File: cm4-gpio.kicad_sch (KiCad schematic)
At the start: 28 parts, among them J1 B2B-PH-SM4-TB_LF__SN_, J5 Conn_02x05_Odd_Even, J6 USB4105-GF-A, U1 MP2624GL-P, U2 MP3423GG-P

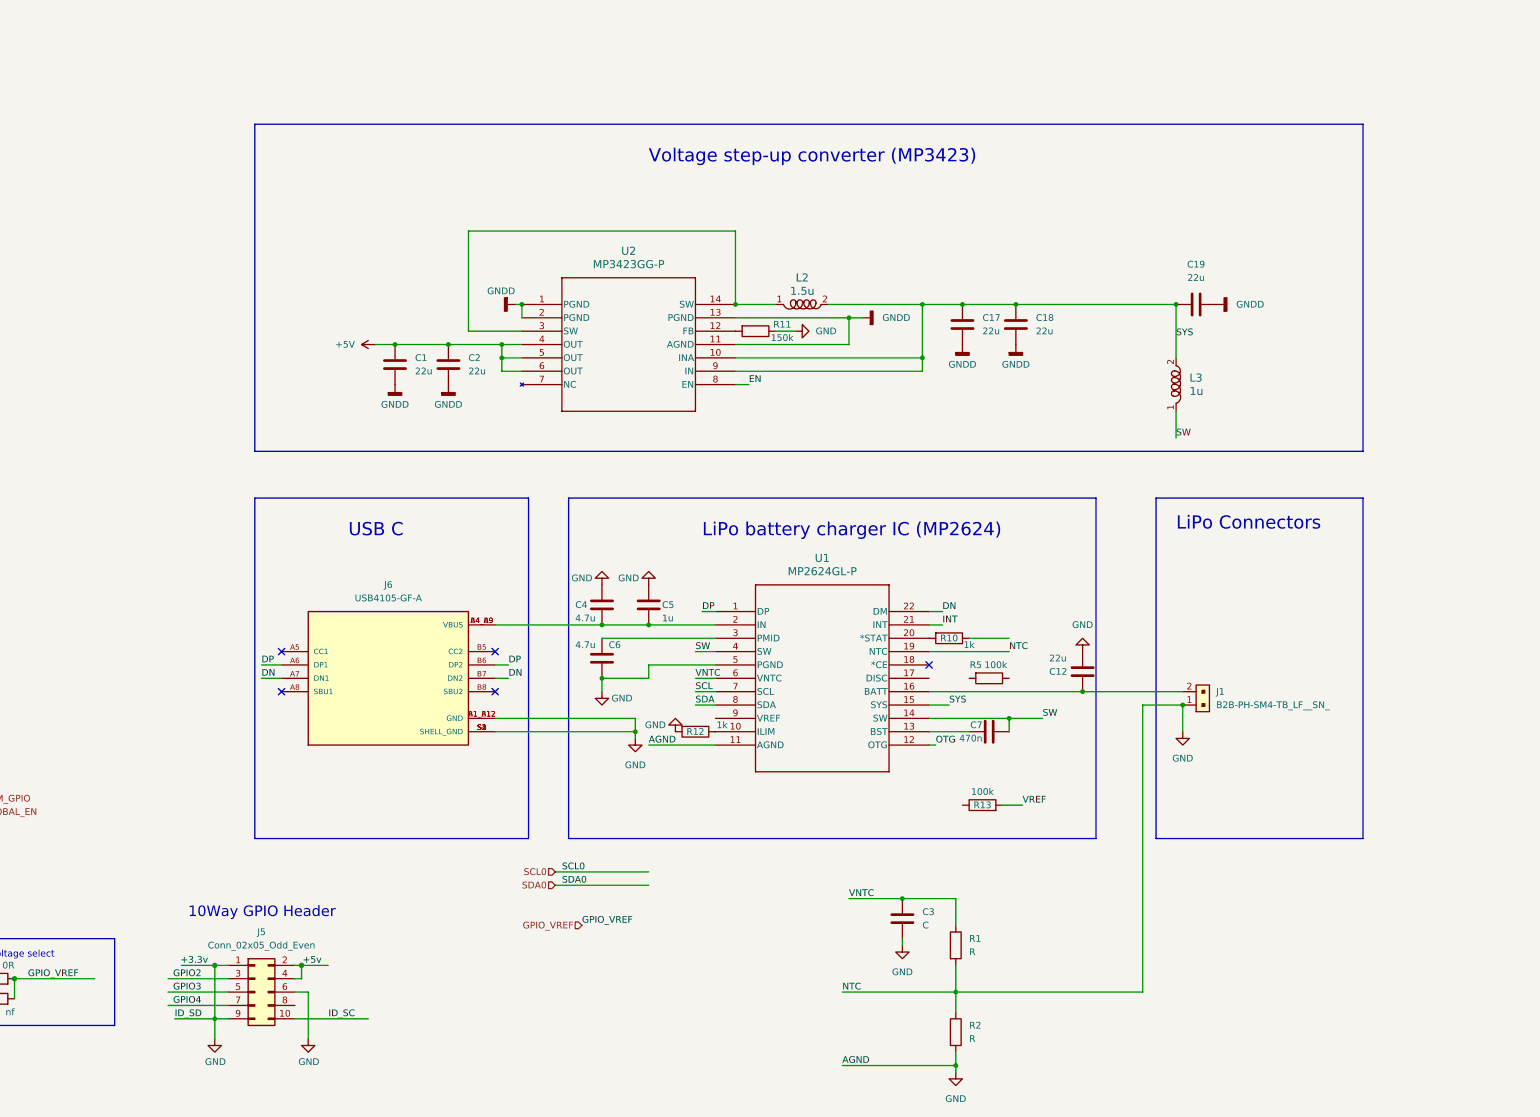
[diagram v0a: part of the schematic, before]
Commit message: -
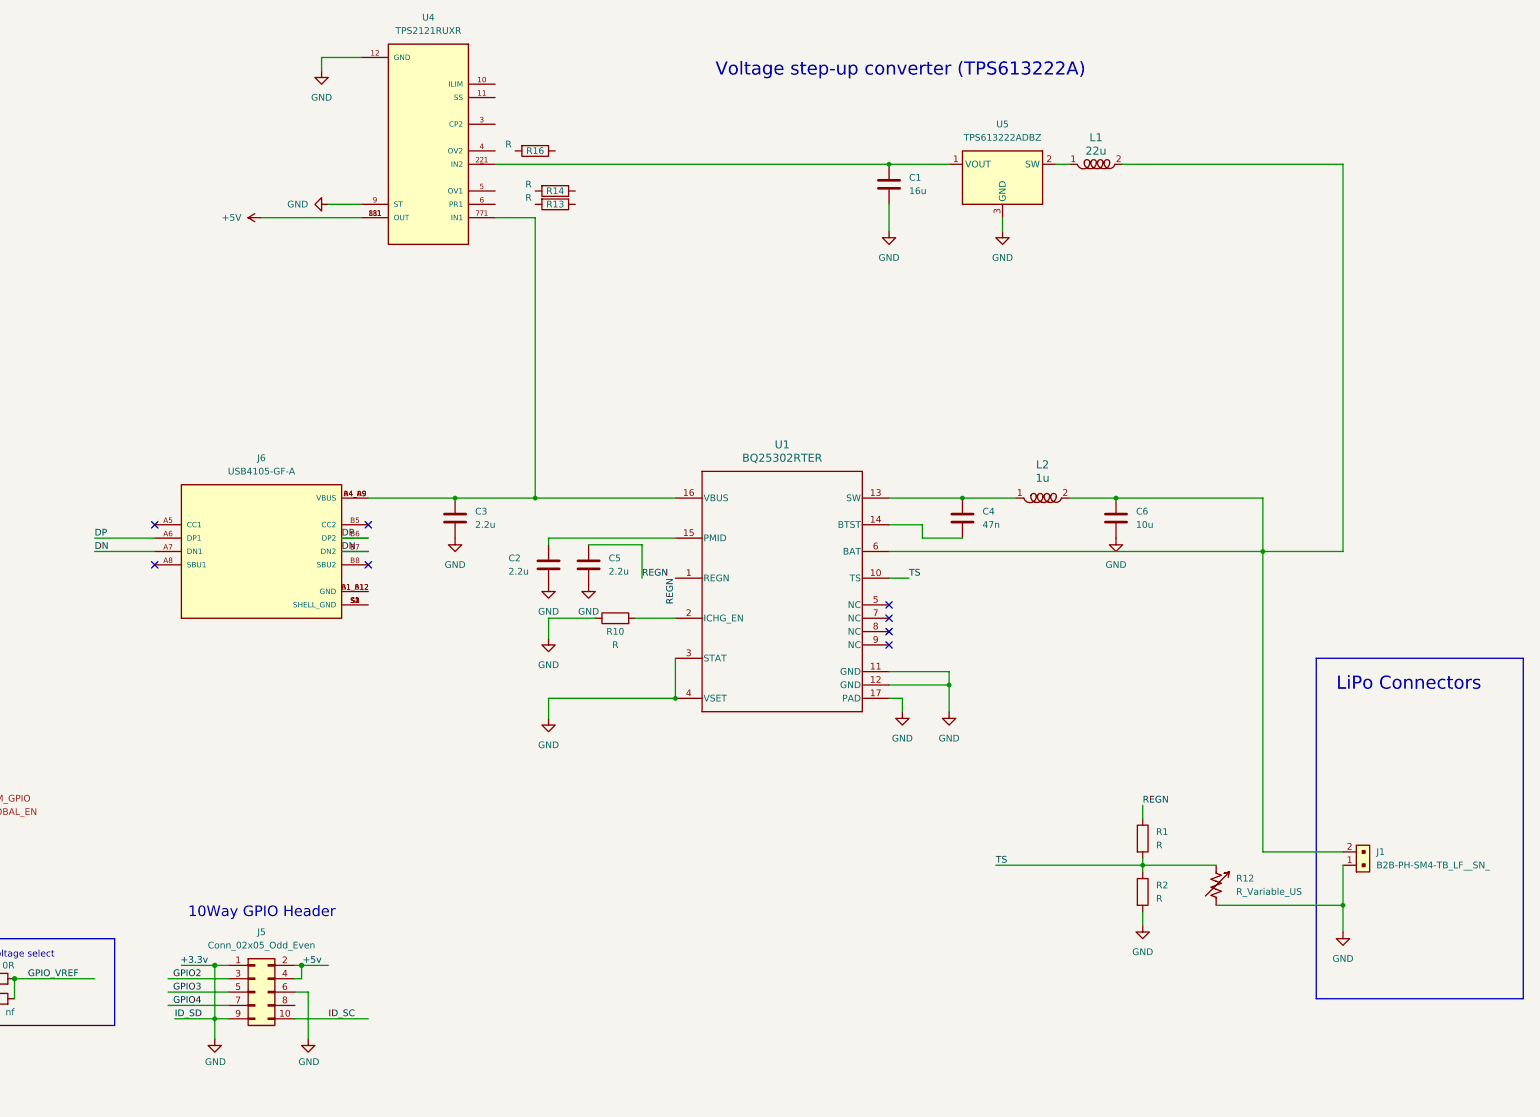
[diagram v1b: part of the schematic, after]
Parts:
- removed C12, C17, C18, C19: 22u, symbol Device:C
- removed C7: 470n, symbol Device:C
- removed L3: 1u, digikey-footprints:Inductor_13R106C, symbol dk_Fixed-Inductors:13R106C
- removed R11: 150k, symbol Device:R
- removed R12: 1k, symbol Device:R
- removed R5: 100k, symbol Device:R
- removed U1: MP2624GL-P, QFN-22_MP2624_MNP, symbol MP2624:MP2624GL-P
- removed U2: MP3423GG-P, QFN14_MP3423_MNP, symbol MP3423:MP3423GG-P
- added L1: 22u, digikey-footprints:Inductor_13R106C, symbol dk_Fixed-Inductors:13R106C
- added R12: R_Variable_US, symbol Device:R_Variable_US
- added R14, R16: R, symbol Device:R
- added U1: BQ25302RTER, RTE0016C, symbol BQ25302:BQ25302RTER
- added U4: TPS2121RUXR, IC_TPS2121RUXR, symbol TPS2121RUXR:TPS2121RUXR
- added U5: TPS613222ADBZ, Package_TO_SOT_SMD:SOT-23, symbol Regulator_Switching:TPS613222ADBZ
- C1: value 22u -> 16u
- C2: value 22u -> 2.2u
- C3: value C -> 2.2u
- C4: value 4.7u -> 47n
- C5: value 1u -> 2.2u
- C6: value 4.7u -> 10u
- L2: value 1.5u -> 1u
- R10: value 1k -> R
- R13: value 100k -> R
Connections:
- net GNDD is gone; now on net GND: C1.2, C2.2
- net SYS is gone; now on an unnamed net: L2.2
- net +5V: now also U4.1 (OUT), U4.1_1 (OUT), U4.8 (OUT), U4.8_1 (OUT); no longer C1.1, C2.1
- net GND: now also C5.2, R10.1, R12.2, U1.11 (GND), U1.12 (GND), U1.17 (PAD), U1.3 (STAT), U1.4 (VSET), U4.12 (GND), U4.9 (ST), U5.3 (GND); no longer C4.1, C5.1, J6.A1_B12 (GND), J6.B1_A12 (GND), J6.S1 (SHELL_GND), J6.S2 (SHELL_GND), J6.S3 (SHELL_GND), J6.S4 (SHELL_GND), R1.2, R2.1
- net at C6.1: now also J1.2, L1.2, U1.6 (BAT)
- net at R10.2: now also U1.2 (ICHG_EN)
- net at L2.1: now also C4.1, U1.13 (SW)
- net at J6.A4_B9 (VBUS), J6.B4_A9 (VBUS): now also C3.1, U1.16 (VBUS), U4.7 (IN1), U4.7_1 (IN1); no longer C4.2, C5.2
- net VNTC renamed REGN
- net REGN: now also C5.1, U1.1 (REGN); no longer C3.1
- net VREF: no longer names the net of R13.2
- new net: C4.2, U1.14 (BTST)
- new net: C1.1, U4.2 (IN2), U4.2_1 (IN2), U5.1 (VOUT)
- new net: L1.1, U5.2 (SW)
- new net: C2.1, U1.15 (PMID)
- new net: J6.A1_B12 (GND), J6.B1_A12 (GND)
- new net: J6.S1 (SHELL_GND), J6.S2 (SHELL_GND), J6.S3 (SHELL_GND), J6.S4 (SHELL_GND)
- new net TS: R1.2, R12.1, R2.1, U1.10 (TS)
- no-connect marks 65 -> 68
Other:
- note added: "Voltage step-up converter (TPS613222A)"
- note removed: "LiPo battery charger IC (MP2624)"
- note removed: "USB C"
- note removed: "Voltage step-up converter (MP3423)"
- moved on the sheet: J1, J6

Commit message: -
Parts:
- removed R12: R_Variable_US, symbol Device:R_Variable_US
- added C7: NTCLE101E3C90173, CAP_E3C90173_VIS, symbol thermistor:NTCLE101E3C90173
- added C8: 16u, symbol Device:C
- added J2, J7: B2B-PH-SM4-TB_LF__SN_, digikey-footprints:PinHeader_1x2_P2mm, symbol dk_Rectangular-Connectors-Headers-Male-Pins:B2B-PH-SM4-TB_LF__SN_
- added R11, R12, R15, R17, R19, R5: R, symbol Device:R
- R1: value R -> 4.527
- R10: value R -> 20k
- R2: value R -> 23.26
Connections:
- net GND: now also J6.A1_B12 (GND), J6.B1_A12 (GND), J6.S1 (SHELL_GND), J6.S2 (SHELL_GND), J6.S3 (SHELL_GND), J6.S4 (SHELL_GND), R14.2, R16.2, C8.2, J2.1, J7.1, R12.2, R17.1, R5.2
- net TS: now also C7.1
- net at L2.1, U1.13 (SW): now also C4.2; no longer C4.1
- net at U1.14 (BTST): now also C4.1; no longer C4.2
- net at U4.10 (ILIM): now also R5.1
- net at U4.11 (SS): now also C8.1
- net IN2: now reaches C1.1, U4.2 (IN2), U4.2_1 (IN2), U5.1 (VOUT)
- net IN2: now also R11.1, R15.1
- net CP2: now reaches U4.3 (CP2)
- net CP2: now also R11.2, R12.1
- net OV2: now reaches U4.4 (OV2)
- net OV2: now also R16.1, R15.2
- net OV1: now reaches U4.5 (OV1)
- net OV1: now also R17.2, R19.1
- net PR1: now reaches U4.6 (PR1)
- net PR1: now also R13.2, R14.1
- net IN1: now reaches C3.1, J6.A4_B9 (VBUS), J6.B4_A9 (VBUS), U1.16 (VBUS), U4.7 (IN1), U4.7_1 (IN1)
- net IN1: now also R13.1, R19.2
- net BAT+: now reaches C6.1, L1.2, L2.2, U1.6 (BAT)
- net BAT+: no longer J1.2
- net +5V: no longer names the net of U4.1 (OUT), U4.1_1 (OUT), U4.8 (OUT), U4.8_1 (OUT)
- new net BAT-: C7.2
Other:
- note added: "LiPo charge managment controller"
- note added: "Temperature Sensing Circuit"
- note added: "USB C Charging Port"
- moved on the sheet: C1, C2, C3, C4, C5, C6, J1, J5, J6, L1, L2, Module1A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

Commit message: schematic complete
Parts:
- removed C8: 16u, symbol Device:C
- removed J2, J7: B2B-PH-SM4-TB_LF__SN_, digikey-footprints:PinHeader_1x2_P2mm, symbol dk_Rectangular-Connectors-Headers-Male-Pins:B2B-PH-SM4-TB_LF__SN_
- removed J5: Conn_02x05_Odd_Even, Connector_PinHeader_2.54mm:PinHeader_2x05_P2.54mm_Vertical, symbol Connector_Generic:Conn_02x05_Odd_Even
- removed R11, R12, R13, R14, R15, R16, R17, R19: R, symbol Device:R
- removed R6: 0R, Resistor_SMD:R_0805_2012Metric_Pad1.15x1.40mm_HandSolder, symbol Device:R
- removed R9: nf, Resistor_SMD:R_0805_2012Metric_Pad1.15x1.40mm_HandSolder, symbol Device:R
- removed U4: TPS2121RUXR, IC_TPS2121RUXR, symbol TPS2121RUXR:TPS2121RUXR
- added D1: CDBA340-HF, Diode_SMD:D_SMA, symbol Diode:CDBA340-HF
- added J1: DNP, Connector_PinHeader_2.54mm:PinHeader_1x10_P2.54mm_Vertical, symbol Connector_Generic:Conn_01x10
- added Q1: DMP3013SFV, Package_SON:Diodes_PowerDI3333-8, symbol Transistor_FET:DMP3013SFV
- C2: value 2.2u -> 10u
- R5: value R -> 1
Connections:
- net BAT- is gone; now on net GND: C7.2
- net IN2 is gone; now on net +5V: C1.1, U5.1 (VOUT)
- net GND: now also R5.1, J1.2 (Pin_2); no longer Module1.75 (SD_PWR_ON), Module1.84 (+3.3v_(Output)), Module1.86 (+3.3v_(Output)), R5.2
- net GPIO7: now reaches Module1.37 (GPIO7)
- net GPIO7: now also J1.9 (Pin_9)
- net GPIO11: now reaches Module1.38 (GPIO11)
- net GPIO11: now also J1.7 (Pin_7)
- net GPIO8: now reaches Module1.39 (GPIO8)
- net GPIO8: now also J1.8 (Pin_8)
- net GPIO9: now reaches Module1.40 (GPIO9)
- net GPIO9: now also J1.6 (Pin_6)
- net GPIO10: now reaches Module1.44 (GPIO10)
- net GPIO10: now also J1.5 (Pin_5)
- net GPIO15: now reaches Module1.51 (GPIO15)
- net GPIO15: now also J1.4 (Pin_4)
- net GPIO14: now reaches Module1.55 (GPIO14)
- net GPIO14: now also J1.3 (Pin_3)
- net nRPIBOOT: now reaches Module1.93 (nRPIBOOT)
- net nRPIBOOT: now also J1.10 (Pin_10)
- net PMID: now reaches C2.1, U1.15 (PMID)
- net PMID: now also Q1.1 (S), Q1.2 (S), Q1.3 (S)
- net at J1.2: now also C6.1, L2.2, U1.6 (BAT), Q1.5 (D)
- net +1.8v renamed +1.8V
- net +5v renamed +5V
- removed net BAT+: C6.1, L1.2, L2.2, U1.6 (BAT)
- net EEPROM_nWP: no longer names the net of Module1.20 (EEPROM_nWP)
- net GLOBAL_EN: no longer names the net of Module1.99 (Global_EN)
- net GPIO_VREF renamed +3.3V
- net +3.3V: now also Module1.84 (+3.3v_(Output)), Module1.86 (+3.3v_(Output)), J1.1 (Pin_1)
- net IN1 renamed VBUS
- net VBUS: now also D1.2 (A)
- net nEXTRST: no longer names the net of Module1.100 (nEXTRST)
- new net: D1.1 (K), Q1.4 (G), R5.2
- new net VSYS: L1.2
- no-connect marks 68 -> 64
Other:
- note added: "GPIO Header"
- note added: "LiPo Connector"
- note added: "SPI0_CE0"
- note added: "SPI0_CE1"
- note added: "SPI0_CLK"
- note added: "SPI0_MISO"
- note added: "SPI0_MOSI"
- note added: "UART0_RXD"
- note added: "UART0_TXD"
- note added: "Voltage step-up converter"
- note added: "nBOOT"
- note removed: "10Way GPIO Header"
- note removed: "GPIO Voltage select"
- note removed: "LiPo Connectors"
- note removed: "Voltage step-up converter (TPS613222A)"
- moved on the sheet: C1, C3, C4, C5, C6, C7, J1, J6, L1, L2, Module1A, R1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
